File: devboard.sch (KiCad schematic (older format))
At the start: 48 parts, among them J1 USB_B, K1 HF3FA-012-ZTF, K2 HF3FA-012-ZTF

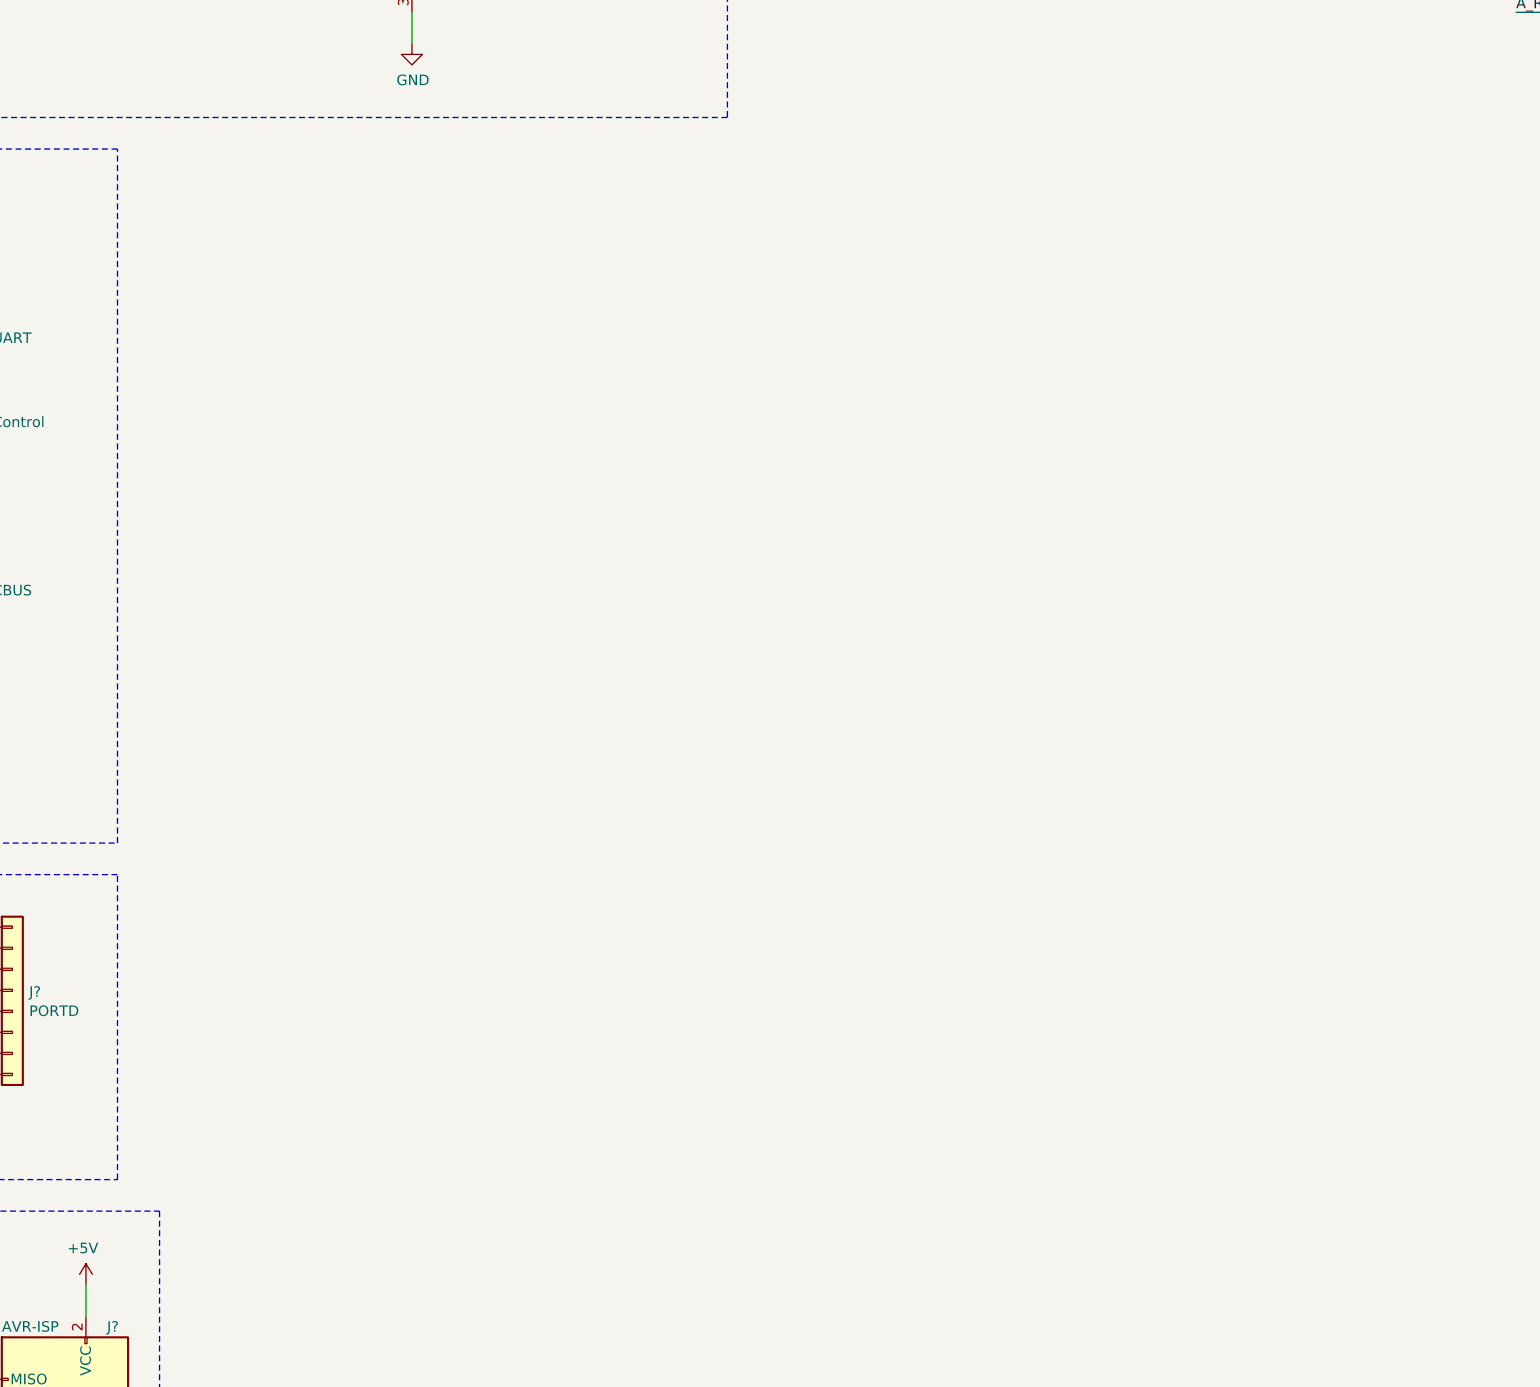
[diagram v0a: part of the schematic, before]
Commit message: LED
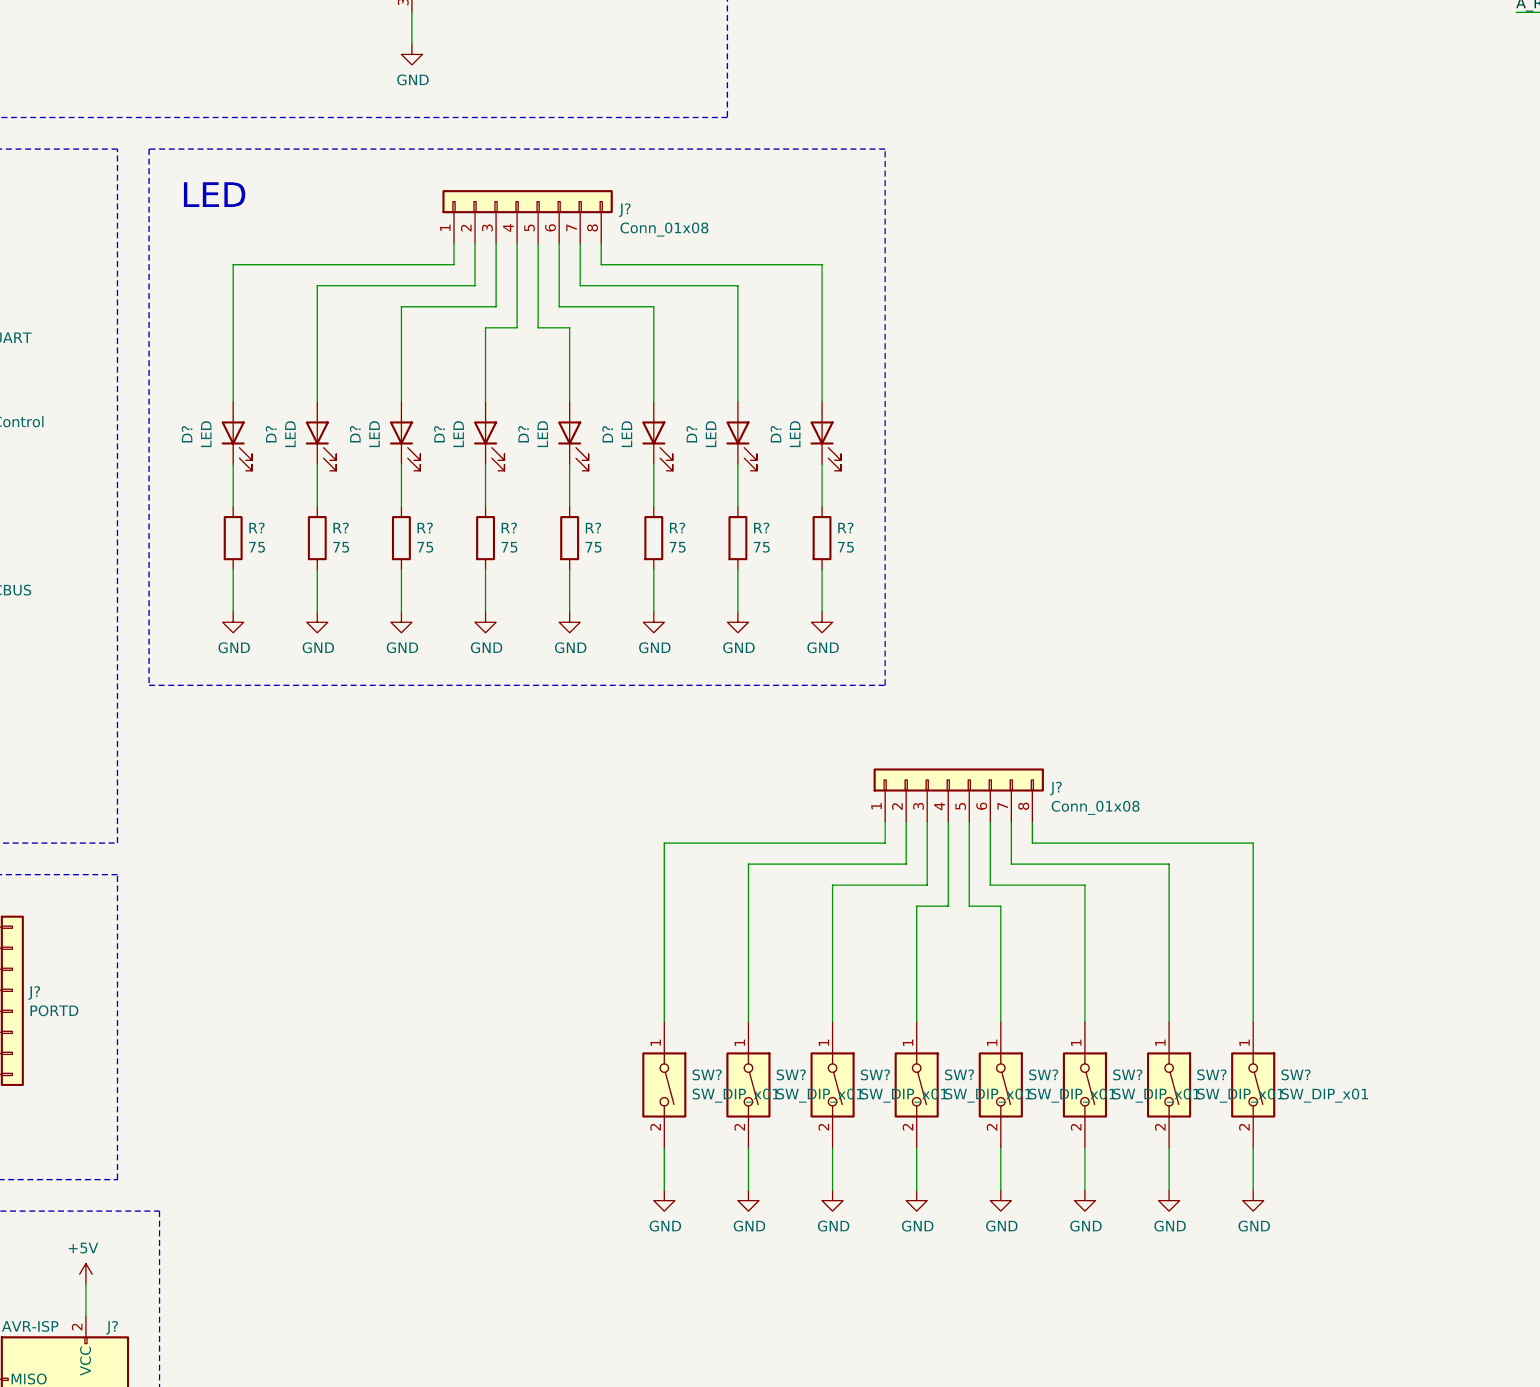
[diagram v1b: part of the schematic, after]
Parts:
- added D? (x8): LED, symbol Device:LED
- added J? (x2): Conn_01x08, symbol Connector_Generic:Conn_01x08
- added R? (x8): 75, symbol Device:R
- added SW? (x8): SW_DIP_x01, symbol Switch:SW_DIP_x01
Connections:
- net GND: now also R?.2, R?.2, R?.2, R?.2, R?.2, R?.2, R?.2, R?.2, SW?.2, SW?.2, SW?.2, SW?.2, SW?.2, SW?.2, SW?.2, SW?.2
- new net: D?.1 (K), R?.1 (x8)
- new net: D?.2 (A), J?.2 (Pin_2)
- new net: D?.2 (A), J?.1 (Pin_1)
- new net: D?.2 (A), J?.3 (Pin_3)
- new net: D?.2 (A), J?.4 (Pin_4)
- new net: D?.2 (A), J?.5 (Pin_5)
- new net: D?.2 (A), J?.6 (Pin_6)
- new net: D?.2 (A), J?.7 (Pin_7)
- new net: D?.2 (A), J?.8 (Pin_8)
- new net: J?.1 (Pin_1), SW?.1
- new net: J?.2 (Pin_2), SW?.1
- new net: J?.3 (Pin_3), SW?.1
- new net: J?.4 (Pin_4), SW?.1
- new net: J?.5 (Pin_5), SW?.1
- new net: J?.6 (Pin_6), SW?.1
- new net: J?.7 (Pin_7), SW?.1
- new net: J?.8 (Pin_8), SW?.1
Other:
- note added: "LED"

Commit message: buttons in progress
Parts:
- removed J?: Conn_01x08, symbol Connector_Generic:Conn_01x08
- removed SW? (x8): SW_DIP_x01, symbol Switch:SW_DIP_x01
- added C? (x12): 100n, symbol Device:C
- added J?: DB Buttons, symbol Connector_Generic:Conn_01x04
- added J?: NDB Buttons, symbol Connector_Generic:Conn_01x04
- added R? (x12): 4k7, symbol Device:R
- added R? (x12): 330, symbol Device:R
- added SW?: B1, symbol Switch:SW_Push
- added SW?: B2, symbol Switch:SW_Push
- added SW?: B3, symbol Switch:SW_Push
- added SW?: B4, symbol Switch:SW_Push
- added SW?: B5, symbol Switch:SW_Push
- added SW?: B6, symbol Switch:SW_Push
- added SW?: B7, symbol Switch:SW_Push
- added SW?: B8, symbol Switch:SW_Push
- added SW?: Switches, symbol Switch:SW_DIP_x08
- J?: value Conn_01x08 -> LED
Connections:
- net +5V: now also R?.1, R?.1, R?.1, R?.1, R?.1, R?.1, R?.1, R?.1, R?.1, R?.1, R?.1, R?.1
- net GND: now also C?.2, C?.2, C?.2, C?.2, C?.2, C?.2, C?.2, C?.2, C?.2, C?.2, C?.2, C?.2, R?.2, R?.2, R?.2, R?.2, SW?.10, SW?.11, SW?.12, SW?.13, SW?.14, SW?.15, SW?.16, SW?.2, SW?.2, SW?.2, SW?.2, SW?.9
- new net: R?.1, SW?.2 (x4)
- new net: R?.2, SW?.1
- new net: R?.2, SW?.2
- new net: R?.2, SW?.3
- new net: R?.2, SW?.4
- new net: R?.2, SW?.5
- new net: R?.2, SW?.6
- new net: R?.2, SW?.7
- new net: R?.2, SW?.8
- new net B1: C?.1, J?.1 (Pin_1), R?.2, SW?.1
- new net B2: C?.1, J?.2 (Pin_2), R?.2, SW?.1
- new net B3: C?.1, J?.3 (Pin_3), R?.2, SW?.1
- new net B4: C?.1, J?.4 (Pin_4), R?.2, SW?.1
- new net B5: J?.1 (Pin_1), SW?.1
- new net B6: J?.2 (Pin_2), SW?.1
- new net B7: J?.3 (Pin_3), SW?.1
- new net B8: J?.4 (Pin_4), SW?.1
- new net S1: C?.1, R?.1, R?.2
- new net S2: C?.1, R?.1, R?.2
- new net S3: C?.1, R?.1, R?.2
- new net S4: C?.1, R?.1, R?.2
- new net S5: C?.1, R?.1, R?.2
- new net S6: C?.1, R?.1, R?.2
- new net S7: C?.1, R?.1, R?.2
- new net S8: C?.1, R?.1, R?.2
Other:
- note added: "CPU"
- note added: "Debounced buttons"
- note added: "Non-debounced buttons"
- moved on the sheet: C?, D?, J?, L?, R?, U?
